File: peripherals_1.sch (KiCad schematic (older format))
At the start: 31 parts, among them J1 Micro_SD_Card_Det, J4 JTAG, J5 0821-1X1T-43-F, U1 TXS0108EPW, U6 PCA9546AD, U8 74AC125, U9 TPS2051B

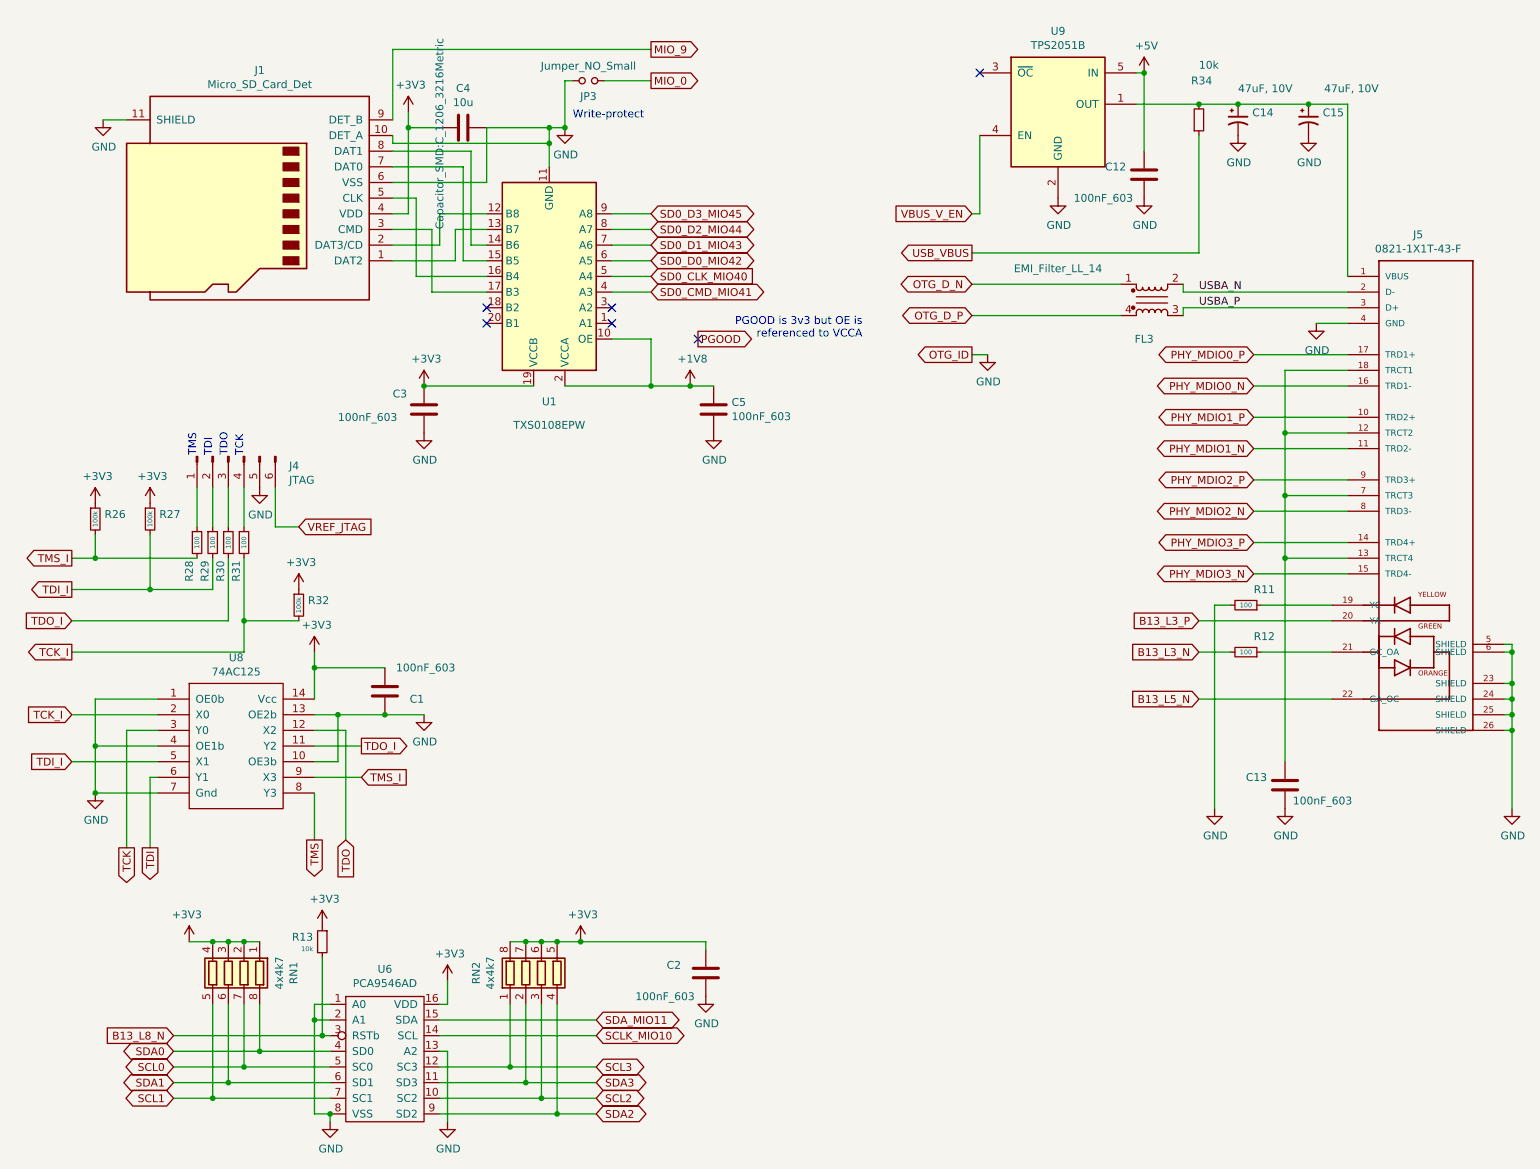
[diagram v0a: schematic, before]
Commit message: WIP: (save)
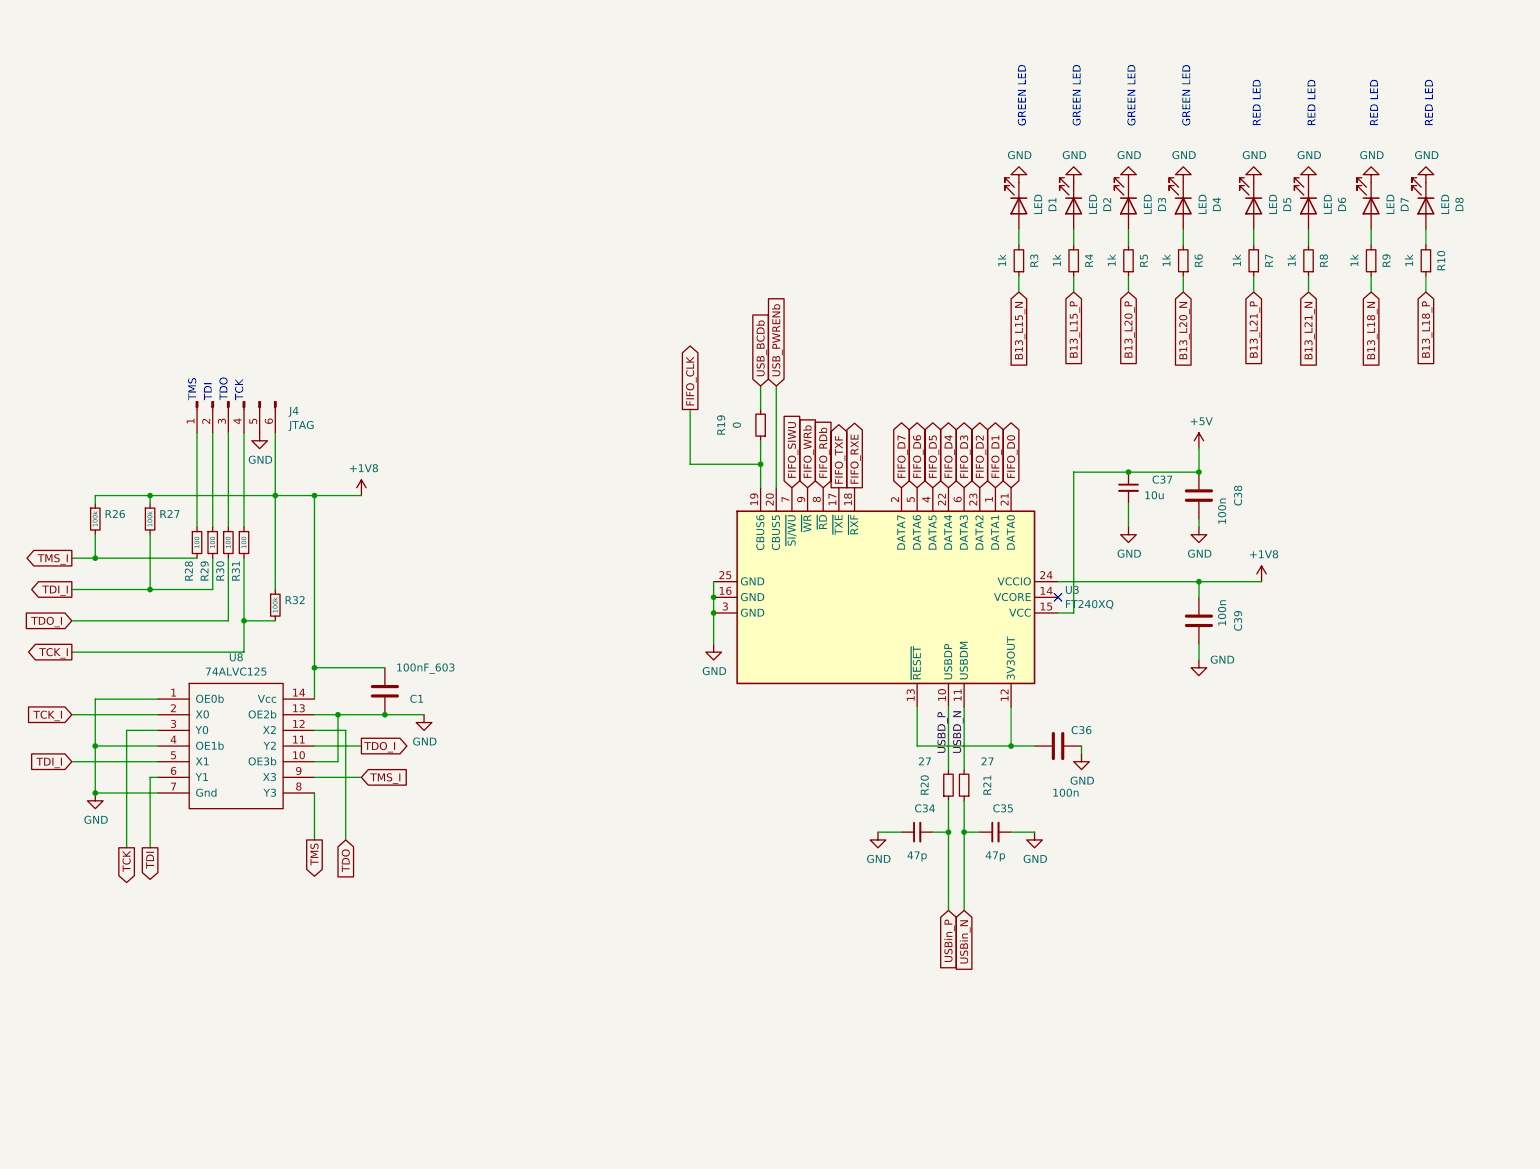
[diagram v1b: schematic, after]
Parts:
- removed C12, C13, C2, C3, C5: 100nF_603, Capacitor_SMD:C_0603_1608Metric, symbol fmc:100nF_603
- removed C14, C15: 47uF, 10V, Capacitor_SMD:C_1206_3216Metric, symbol Device:CP1_Small
- removed C4: 10u, Capacitor_SMD:C_1206_3216Metric, symbol Device:C
- removed FL3: EMI_Filter_LL_14, proj_footprints:WE_CNSW, symbol fmc:EMI_Filter_LL_14
- removed J1: Micro_SD_Card_Det, proj_footprints:microSD_HC_Hirose_DM3D-SF_smaller_crtyd, symbol Connector:Micro_SD_Card_Det
- removed J5: 0821-1X1T-43-F, proj_footprints:BEL_0821-1X1T-43-F, symbol fmc:0821-1X1T-43-F
- removed JP3: Jumper_NO_Small, Connector_PinHeader_2.54mm:PinHeader_1x02_P2.54mm_Vertical, symbol Device:Jumper_NO_Small
- removed R11, R12: 100, Resistor_SMD:R_0603_1608Metric, symbol Device:R_Small
- removed R13, R34: 10k, Resistor_SMD:R_0603_1608Metric, symbol trigbox:R10k
- removed RN1, RN2: 4x4k7, Resistor_SMD:R_Array_Convex_4x0603, symbol Device:R_Pack04
- removed U1: TXS0108EPW, Package_SO:TSSOP-20_4.4x6.5mm_P0.65mm, symbol Logic_LevelTranslator:TXS0108EPW
- removed U6: PCA9546AD, Package_SO:SOIC-16_3.9x9.9mm_P1.27mm, symbol fmc:PCA9546AD
- removed U9: TPS2051B, Package_TO_SOT_SMD:SOT-23-5, symbol fmc:TPS2051B
- added C34, C35: 47p, Capacitor_SMD:C_0603_1608Metric, symbol Device:C_Small
- added C36, C38, C39: 100n, Capacitor_SMD:C_0603_1608Metric, symbol fmc:100nF_603
- added C37: 10u, Capacitor_SMD:C_1206_3216Metric, symbol Device:C_Small
- added D1, D2, D3, D4, D5, D6, D7, D8: LED, LED_SMD:LED_0603_1608Metric, symbol Device:LED
- added R10, R3, R4, R5, R6, R7, R8, R9: 1k, Resistor_SMD:R_0603_1608Metric, symbol Device:R_Small
- added R19: 0, Resistor_SMD:R_0402_1005Metric, symbol Device:R_Small
- added R20, R21: 27, Resistor_SMD:R_0603_1608Metric, symbol Device:R_Small
- added U3: FT240XQ, Package_DFN_QFN:QFN-24-1EP_4x4mm_P0.5mm_EP2.6x2.6mm, symbol fmc:FT240XQ
- U8: value 74AC125 -> 74ALVC125
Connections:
- net +3V3 is gone; now on net +1V8: C1.2, R26.1, R27.1, R32.1, U8.14 (Vcc)
- net VREF_JTAG is gone; now on net +1V8: J4.6 (Pin_6)
- net +1V8: now also C39.2, U3.24 (VCCIO)
- net +5V: now also C37.1, C38.2, U3.15 (VCC)
- net GND: now also C34.1, C35.2, C36.1, C37.2, C38.1, C39.1, D1.1 (K), D2.1 (K), D3.1 (K), D4.1 (K), D5.1 (K), D6.1 (K), D7.1 (K), D8.1 (K), U3.16 (GND), U3.25 (GND), U3.3 (GND)
- new net: C36.2, U3.12 (3V3OUT), U3.13 (~RESET)
- new net: D1.2 (A), R3.2
- new net: D2.2 (A), R4.2
- new net: D3.2 (A), R5.2
- new net: D4.2 (A), R6.2
- new net: D5.2 (A), R7.2
- new net: D6.2 (A), R8.2
- new net: D7.2 (A), R9.2
- new net: D8.2 (A), R10.2
- new net B13_L15_N: R3.1
- new net B13_L15_P: R4.1
- new net B13_L18_N: R9.1
- new net B13_L18_P: R10.1
- new net B13_L20_N: R6.1
- new net B13_L20_P: R5.1
- new net B13_L21_N: R8.1
- new net B13_L21_P: R7.1
- new net FIFO_CLK: R19.1, U3.19 (CBUS6)
- new net FIFO_D0: U3.21 (DATA0)
- new net FIFO_D1: U3.1 (DATA1)
- new net FIFO_D2: U3.23 (DATA2)
- new net FIFO_D3: U3.6 (DATA3)
- new net FIFO_D4: U3.22 (DATA4)
- new net FIFO_D5: U3.4 (DATA5)
- new net FIFO_D6: U3.5 (DATA6)
- new net FIFO_D7: U3.2 (DATA7)
- new net FIFO_RDb: U3.8 (~RD)
- new net FIFO_RXE: U3.18 (~RXF)
- new net FIFO_SIWU: U3.7 (~SI/WU)
- new net FIFO_TXF: U3.17 (~TXE)
- new net FIFO_WRb: U3.9 (~WR)
- new net USBD_N: R21.2, U3.11 (USBDM)
- new net USBD_P: R20.2, U3.10 (USBDP)
- new net USB_BCDb: R19.2
- new net USB_PWRENb: U3.20 (CBUS5)
- new net USBin_N: C35.1, R21.1
- new net USBin_P: C34.2, R20.1
- no-connect marks 6 -> 1
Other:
- note added: "GREEN LED"
- note added: "RED LED"
- note removed: "PGOOD is 3v3 but OE is\nreferenced to VCCA"
- note removed: "Write-protect"
- moved on the sheet: J4, R32
